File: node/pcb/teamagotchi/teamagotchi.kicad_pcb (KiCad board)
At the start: 2 copper layers, 2 parts

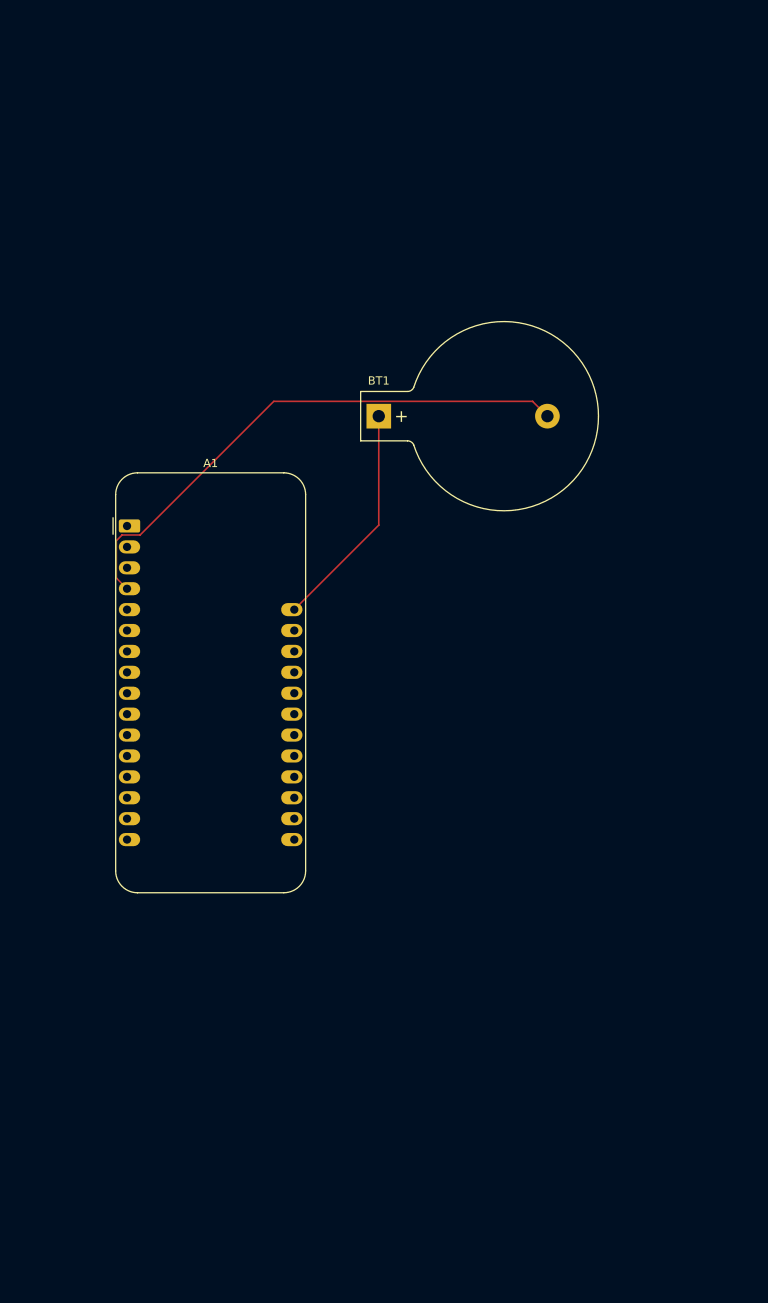
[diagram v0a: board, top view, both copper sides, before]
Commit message: first shot of the pcv
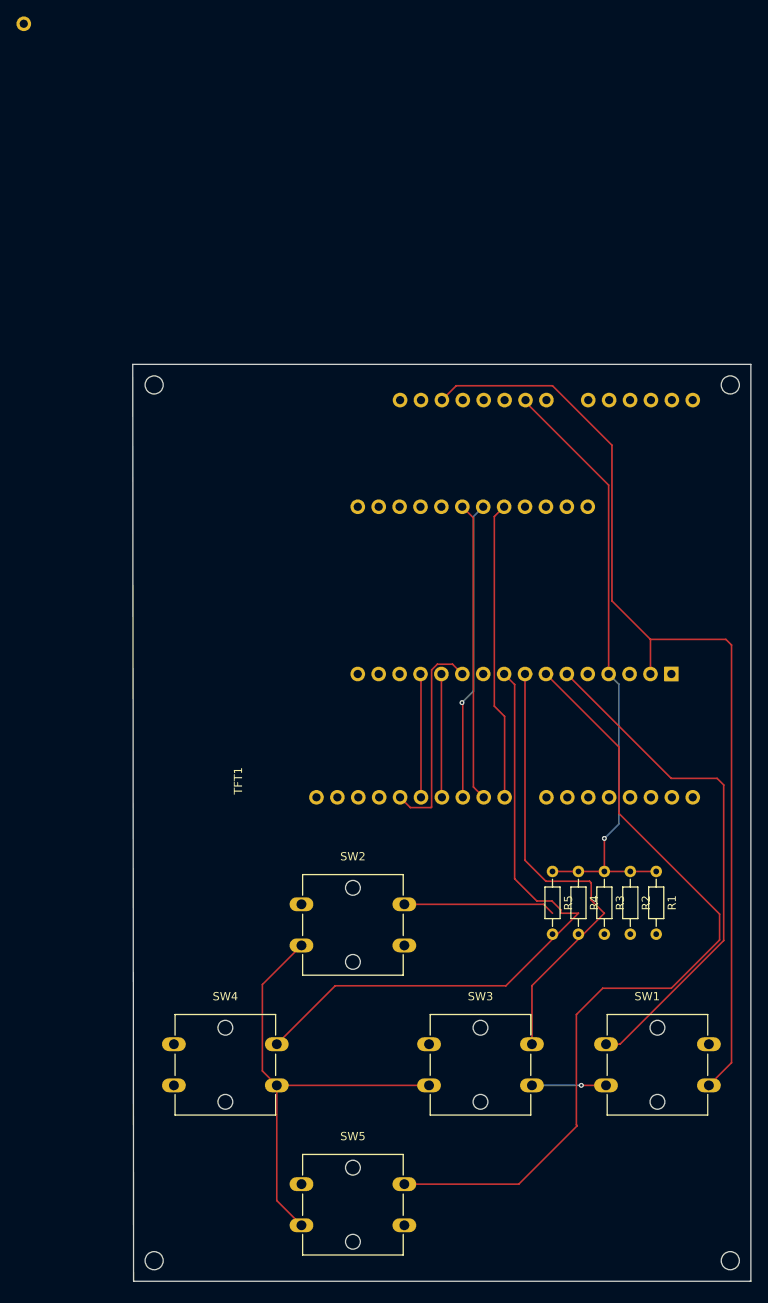
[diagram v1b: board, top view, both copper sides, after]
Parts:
- removed A1: Adafruit_Feather_Generic, Module:Adafruit_Feather
- removed BT1: Battery, Battery:BatteryHolder_Keystone_103_1x20mm
- added R1: R, Resistor_THT:R_Axial_DIN0204_L3.6mm_D1.6mm_P7.62mm_Horizontal, F.Cu at (173.5, 108.3)
- added R2: R, Resistor_THT:R_Axial_DIN0204_L3.6mm_D1.6mm_P7.62mm_Horizontal, F.Cu at (170.3, 108.3)
- added R3: R, Resistor_THT:R_Axial_DIN0204_L3.6mm_D1.6mm_P7.62mm_Horizontal, F.Cu at (167.2, 108.3)
- added R4: R, Resistor_THT:R_Axial_DIN0204_L3.6mm_D1.6mm_P7.62mm_Horizontal, F.Cu at (164.0, 108.3)
- added R5: R, Resistor_THT:R_Axial_DIN0204_L3.6mm_D1.6mm_P7.62mm_Horizontal, F.Cu at (160.9, 108.3)
- added REF**: MountingHole_2.2mm_M2, MountingHole:MountingHole_2.2mm_M2, F.Cu at (182.5, 49.2)
- added REF**: MountingHole_2.2mm_M2, MountingHole:MountingHole_2.2mm_M2, F.Cu at (112.5, 49.2)
- added REF**: MountingHole_2.2mm_M2, MountingHole:MountingHole_2.2mm_M2, F.Cu at (182.5, 155.6)
- added REF**: MountingHole_2.2mm_M2, MountingHole:MountingHole_2.2mm_M2, F.Cu at (112.5, 155.6)
- added SW1: SW_Push, Button_Switch_THT:SW_SPST_Omron_B3F-40xx, F.Cu at (167.4, 129.3)
- added SW2: SW_Push, Button_Switch_THT:SW_SPST_Omron_B3F-40xx, F.Cu at (130.4, 112.3)
- added SW3: SW_Push, Button_Switch_THT:SW_SPST_Omron_B3F-40xx, F.Cu at (145.9, 129.3)
- added SW4: SW_Push, Button_Switch_THT:SW_SPST_Omron_B3F-40xx, F.Cu at (114.9, 129.3)
- added SW5: SW_Push, Button_Switch_THT:SW_SPST_Omron_B3F-40xx, F.Cu at (130.4, 146.3)
- added TFT1: ~, Library:Display-2.8, F.Cu at (126.7, 92.8)
- added U1: 3406, Library:MODULE_3406, B.Cu at (156.2, 74.2)
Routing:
- net Net-(TFT1-3/5V): track 0.00 -> 185.0 mm, vias 0 -> 1
- net Net-(U1-A2/0.04): track 0.00 -> 100.9 mm
- net Net-(U1-A4/0.28): track 0.00 -> 78.4 mm
- net Net-(TFT1-GND): track 0.00 -> 75.3 mm, vias 0 -> 1
- net Net-(A1-GND): track 66.5 -> 0.00 mm
- net Net-(U1-A1/0.03): track 0.00 -> 63.3 mm
- net Net-(U1-A3/0.05): track 0.00 -> 56.6 mm
- net Net-(TFT1-D10/TFT_CS): track 0.00 -> 36.8 mm, vias 0 -> 1
- net Net-(TFT1-D9/TFT_DC): track 0.00 -> 36.4 mm
- net Net-(TFT1-D8/Touch_CS): track 0.00 -> 36.3 mm
- net Net-(A1-VBAT): track 27.8 -> 0.00 mm
- net Net-(TFT1-D13/SCLK): track 0.00 -> 25.5 mm
- net Net-(R5-Pad2): track 0.00 -> 18.5 mm
- net Net-(TFT1-D12/MISO): track 0.00 -> 15.0 mm
- net Net-(TFT1-D11/MOSI): track 0.00 -> 15.0 mm
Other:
- board outline added: 75.1 x 111.4 mm

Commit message: first 1.0 of PCB
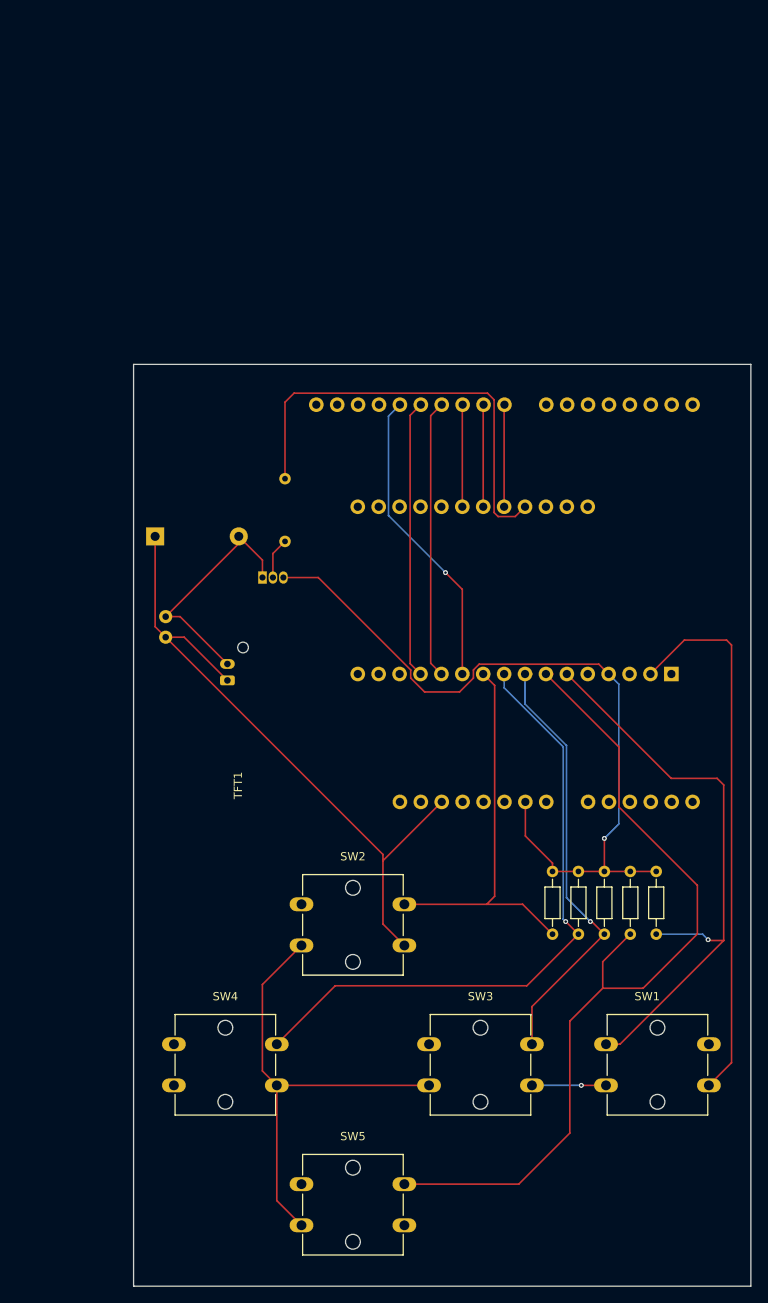
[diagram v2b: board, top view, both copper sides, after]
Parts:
- removed REF** (x4): MountingHole_2.2mm_M2, MountingHole:MountingHole_2.2mm_M2
- added C1: C, Capacitor_THT:C_Disc_D3.0mm_W1.6mm_P2.50mm, B.Cu at (113.9, 79.9)
- added D1: 1N4001, Diode_THT:D_DO-41_SOD81_P10.16mm_Horizontal, B.Cu at (112.6, 67.6)
- added M1: Motor_DC, Connector_Molex:Molex_MicroClasp_55932-0210_1x02_P2.00mm_Vertical, B.Cu at (121.4, 85.1)
- added Q1: BC547, Package_TO_SOT_THT:TO-92_Inline, B.Cu at (125.6, 72.6)
- added R6: R, Resistor_THT:R_Axial_DIN0204_L3.6mm_D1.6mm_P7.62mm_Horizontal, B.Cu at (128.4, 60.6)
- moved TFT1 65.7 mm to (177.9, 51.6)
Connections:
- R5 pad 2: Net-(R5-Pad2) -> Net-(U1-A5/0.29)
- SW2 pad 1: Net-(R5-Pad2) -> Net-(U1-A5/0.29)
- U1 pad 10: unconnected-(U1-A5/0.29-Pad10) -> Net-(U1-A5/0.29)
- U1 pad 22: Net-(TFT1-D9/TFT_DC) -> Net-(TFT1-D10/TFT_CS)
- U1 pad 23: Net-(TFT1-D10/TFT_CS) -> Net-(TFT1-D9/TFT_DC)
- U1 pad 25: unconnected-(U1-P0.16-Pad25) -> Net-(U1-P0.16)
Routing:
- net Net-(U1-P0.16): track 0.00 -> 53.6 mm
- net Net-(U1-A5/0.29): track 0.00 -> 48.5 mm
- net Net-(D1-K): track 185.0 -> 214.8 mm
- net Net-(D1-A): track 0.00 -> 29.5 mm
- net Net-(TFT1-D10/TFT_CS): track 36.8 -> 12.4 mm, vias 1 -> 0
- net Net-(TFT1-D9/TFT_DC): track 36.4 -> 12.4 mm
- net Net-(TFT1-D8/Touch_CS): track 36.3 -> 12.4 mm
- net Net-(Q1-E): track 75.3 -> 96.0 mm
- net Net-(TFT1-D12/MISO): track 15.0 -> 33.9 mm
- net Net-(TFT1-D11/MOSI): track 15.0 -> 33.8 mm
- net Net-(R5-Pad2): track 18.5 -> 0.00 mm
- net Net-(TFT1-D13/SCLK): track 25.5 -> 37.0 mm, vias 0 -> 1
- net Net-(U1-A1/0.03): track 63.3 -> 71.9 mm, vias 0 -> 1
- net Net-(Q1-B): track 0.00 -> 5.00 mm
- net Net-(U1-A2/0.04): track 100.9 -> 104.5 mm
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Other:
- board size 75.1 x 111.4 mm -> 75 x 112 mm
- board text added: "R4"
